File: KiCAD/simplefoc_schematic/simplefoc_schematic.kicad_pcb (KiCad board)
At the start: 2 copper layers, 57.8 x 127.6 mm, 75 parts, among them IC1 TMC6140-Trinamic, J1 Power Supply, J2 Motor Connector, J3 Sensor Connector, J5 Programming Port, J6 UART Port, J7 Servo, Q1 IRLR 2905, Q2 IRLR 2905, Q3 IRLR 2905, Q4 IRLR 2905, Q5 IRLR 2905, Q6 IRLR 2905, SW1 SW_Push, U1 MC7805CDTG, U2 STM32F101CBT6

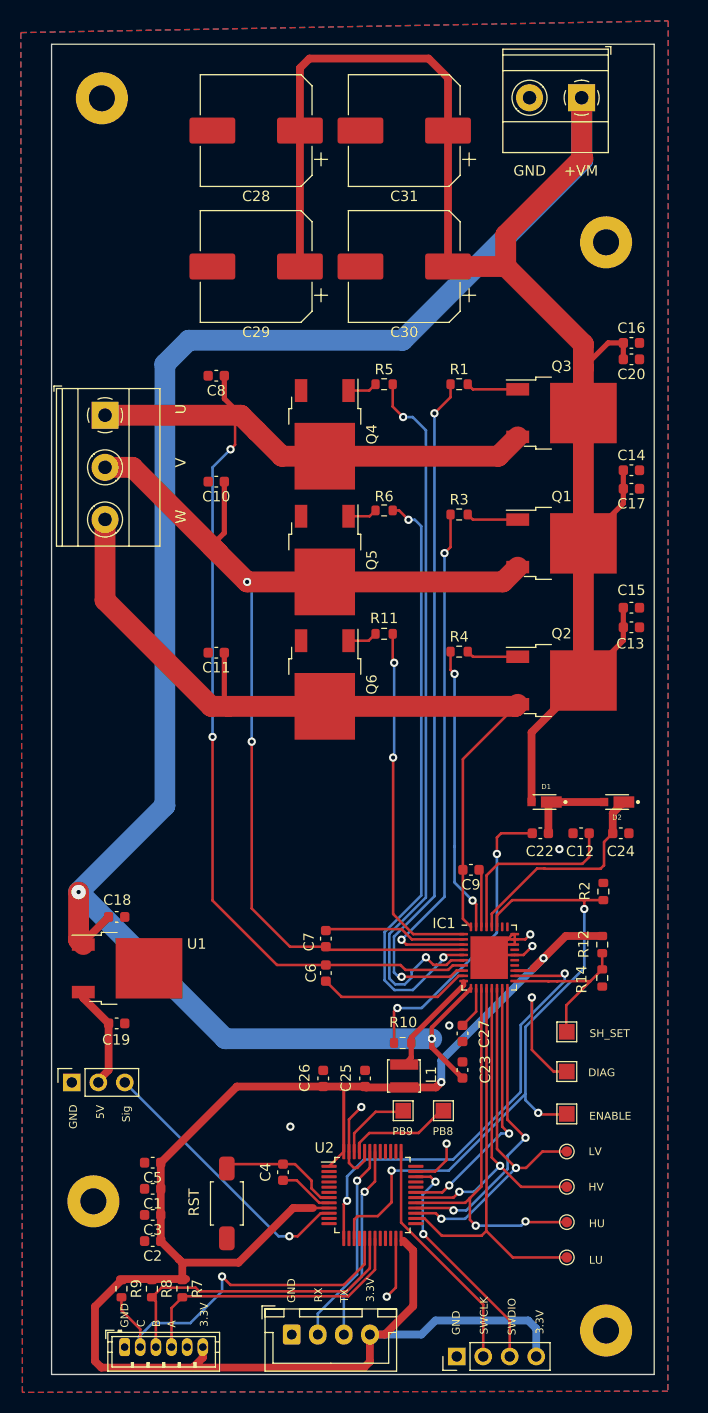
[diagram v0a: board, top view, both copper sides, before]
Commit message: First design of the final small PCB
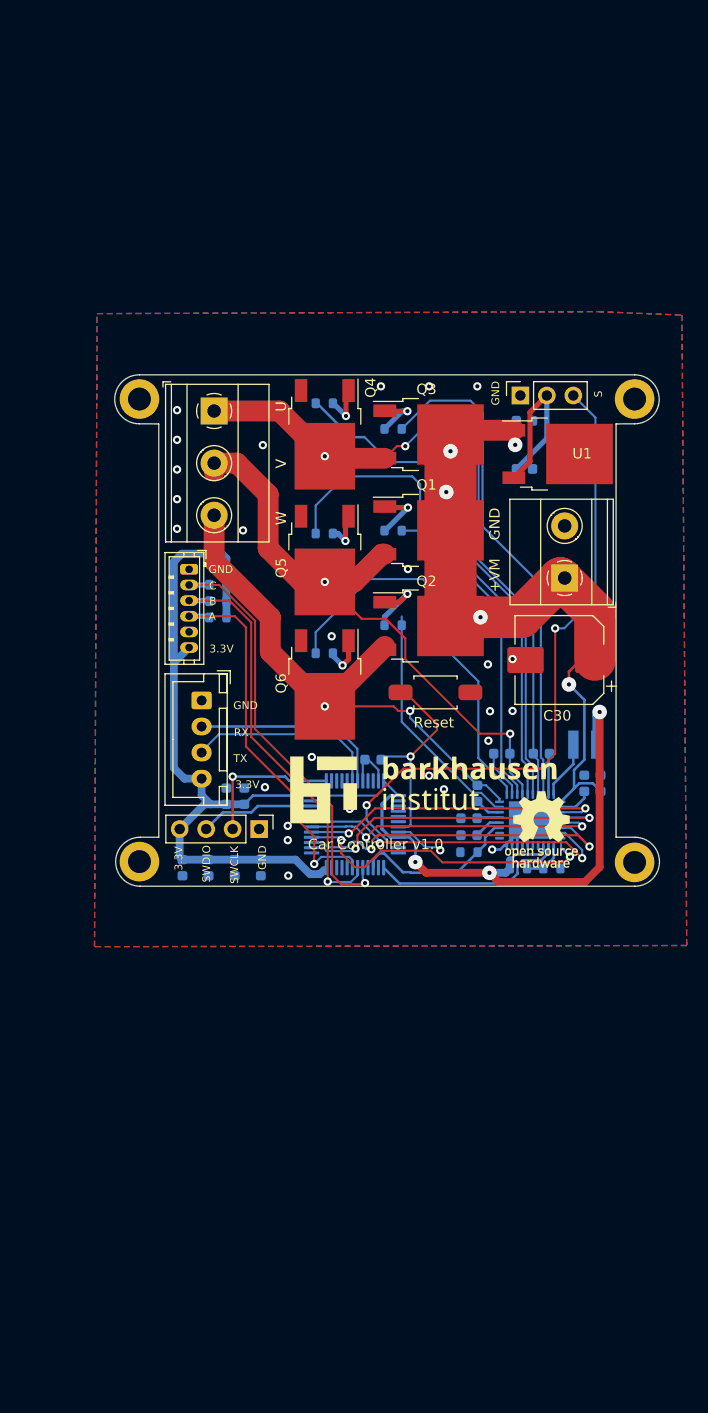
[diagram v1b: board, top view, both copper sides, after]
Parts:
- removed C22: 100nF/35V, Capacitor_SMD:C_0603_1608Metric
- removed C28, C29, C31: 1000uF/25V, Capacitor_SMD:CP_Elec_10x14.3
- removed D1, D2: D_Schottky, Additional_Components:DIODE_MSS1P4-M3_89A
- removed R10: 0R, Resistor_SMD:R_0603_1608Metric
- removed TP1, TP2, TP4, TP5, TP6: TestPoint, TestPoint:TestPoint_Pad_1.5x1.5mm
- removed TP3, TP7, TP8, TP9: TestPoint, TestPoint:TestPoint_Pad_D1.0mm
- added G***: LOGO, LOGO, F.Cu at (103.3, 99.7)
- added G***: LOGO, LOGO, F.Cu at (114.7, 103.5)
- C1, C10, C11, C12, C13, C14, C15, C16, C17, C18, C19, C2, C20, C23, C24, C25, C26, C27, C3, C4, C5, C6, C7, C8, C9, IC1, L1, R1, R11, R12, R14, R2, R3, R4, R5, R6, R7, R8, R9, U2: moved to B.Cu
- C30: value 1000uF/25V -> 220uF/25V; footprint Capacitor_SMD:CP_Elec_10x14.3 -> Capacitor_SMD:CP_Elec_8x10
- H1, H2, H3, H4: footprint MountingHole:MountingHole_2.5mm_Pad -> MountingHole:MountingHole_2.2mm_M2_DIN965_Pad
- moved H4 89.4 mm to (123.6, 62.2)
- moved J7 78.7 mm to (112.7, 61.8)
- moved H2 77.1 mm to (76.1, 62.2)
- moved J3 74.9 mm to (80.9, 78.5), turned to -90 degrees
- moved H3 73.3 mm to (76.1, 106.6)
- moved R9 68.2 mm to (83.7, 80.0), turned to 180 degrees
- moved R8 66.3 mm to (83.7, 81.6), turned to 180 degrees
- moved C19 66.0 mm to (113.1, 68.9)
- moved R7 64.5 mm to (83.7, 83.1), turned to 180 degrees
- moved U1 64.3 mm to (116.3, 67.5)
- moved C18 61.6 mm to (113.1, 64.3)
- moved J6 61.4 mm to (82.1, 91.1), turned to -90 degrees
- moved H1 59.5 mm to (123.6, 106.6)
- moved J5 54.0 mm to (87.6, 103.4), turned to -90 degrees
- moved SW1 53.0 mm to (104.5, 90.3), turned to 180 degrees
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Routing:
- net +BATT: track 324.7 -> 80.2 mm, vias 2 -> 5
- net U: track 120.7 -> 70.5 mm
- net ENABLE: track 63.0 -> 16.1 mm, vias 3 -> 0
- net V: track 105.9 -> 60.1 mm
- net DIAG: track 56.2 -> 18.8 mm, vias 3 -> 0
- net +3.3V: track 171.2 -> 134.8 mm, vias 2 -> 3
- net Servo: track 26.6 -> 62.9 mm, vias 1 -> 2
- net Net-(C22-Pad2): track 28.7 -> 0.00 mm, vias 2 -> 0
- net W: track 80.8 -> 54.2 mm, vias 0 -> 2
- net LOUTU: track 69.6 -> 50.7 mm, vias 2 -> 0
- net GND: track 41.8 -> 23.3 mm, vias 8 -> 27
- net Net-(C24-Pad2): track 20.8 -> 2.66 mm
- net HOUTV: track 48.9 -> 31.1 mm, vias 2 -> 0
- net HOUTU: track 65.8 -> 48.4 mm, vias 2 -> 0
- net Net-(C12-Pad2): track 17.8 -> 2.19 mm
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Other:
- board size 57.8 x 127.6 mm -> 52.3 x 49.1 mm
- board text added: "Car Controller v1.0"
- board text added: "Reset"
- board text added: "S"
- board text removed: "5V"
- board text removed: "DIAG"
- board text removed: "ENABLE"
- board text removed: "HU"
- board text removed: "HV"
- board text removed: "LU"
- board text removed: "LV"
- board text removed: "PB8"
- board text removed: "PB9"
- board text removed: "RST"
- board text removed: "SH_SET"
- board text removed: "Sig"
